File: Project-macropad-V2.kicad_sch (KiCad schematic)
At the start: 50 parts, among them J1 Conn_01x04_Male, SW1 RotaryEncoder_Switch, SW2 SW_Push, SW3 SW_SPDT

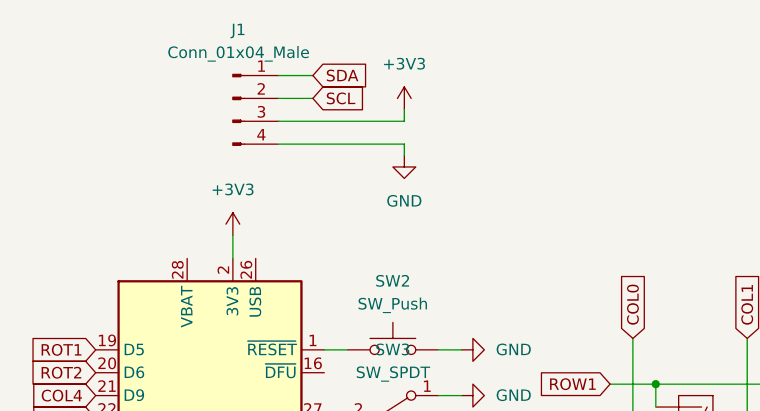
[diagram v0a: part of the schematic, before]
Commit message: Finished PCB
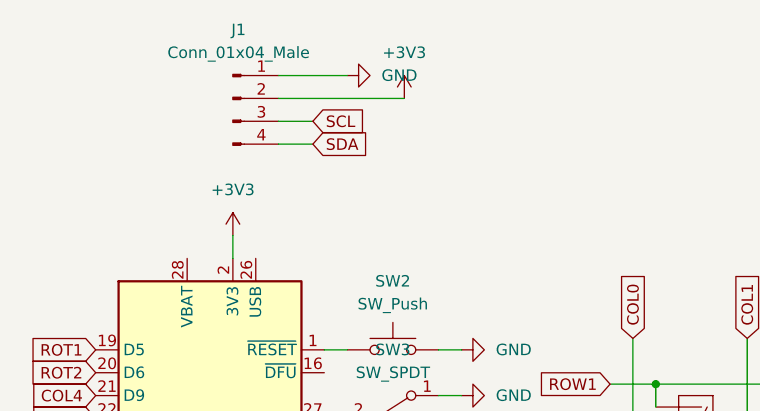
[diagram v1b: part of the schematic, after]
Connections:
- net +3V3: now also J1.2 (Pin_2); no longer J1.3 (Pin_3)
- net GND: now also J1.1 (Pin_1); no longer J1.4 (Pin_4)
- net SCL: now also J1.3 (Pin_3); no longer J1.2 (Pin_2)
- net SDA: now also J1.4 (Pin_4); no longer J1.1 (Pin_1)
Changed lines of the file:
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@@
-    (stroke (width 0) (type default) (color 0 0 0 0))
-  )
-  (wire (pts (xy 82.55 34.29) (xy 82.55 33.02))
     (stroke (width 0) (type default) (color 0 0 0 0))
   )
@@
     (stroke (width 0) (type default) (color 0 0 0 0))
   )
-  (wire (pts (xy 68.58 33.02) (xy 82.55 33.02))
-    (stroke (width 0) (type default) (color 0 0 0 0))
-  )
   (wire (pts (xy 135.89 125.73) (xy 135.89 128.27))
     (stroke (width 0) (type default) (color 0 0 0 0))
@@
     (stroke (width 0) (type default) (color 0 0 0 0))
   )
-  (wire (pts (xy 68.58 25.4) (xy 72.39 25.4))
-    (stroke (width 0) (type default) (color 0 0 0 0))
-  )
   (wire (pts (xy 110.49 78.74) (xy 110.49 76.2))
     (stroke (width 0) (type default) (color 0 0 0 0))
@@
     (stroke (width 0) (type default) (color 0 0 0 0))
   )
+  (wire (pts (xy 68.58 33.02) (xy 72.39 33.02))
+    (stroke (width 0) (type default) (color 0 0 0 0))
+  )
   (wire (pts (xy 115.57 67.31) (xy 109.22 67.31))
     (stroke (width 0) (type default) (color 0 0 0 0))
@@
     (stroke (width 0) (type default) (color 0 0 0 0))
   )
+  (wire (pts (xy 68.58 25.4) (xy 76.2 25.4))
+    (stroke (width 0) (type default) (color 0 0 0 0))
+  )
   (wire (pts (xy 123.19 92.71) (xy 135.89 92.71))
     (stroke (width 0) (type default) (color 0 0 0 0))
@@
     (stroke (width 0) (type default) (color 0 0 0 0))
   )
+  (wire (pts (xy 68.58 27.94) (xy 82.55 27.94))
+    (stroke (width 0) (type default) (color 0 0 0 0))
+  )
   (wire (pts (xy 115.57 128.27) (xy 115.57 125.73))
     (stroke (width 0) (type default) (color 0 0 0 0))
@@
     (stroke (width 0) (type default) (color 0 0 0 0))
   )
-  (wire (pts (xy 68.58 27.94) (xy 72.39 27.94))
-    (stroke (width 0) (type default) (color 0 0 0 0))
-  )
   (wire (pts (xy 128.27 83.82) (xy 121.92 83.82))
     (stroke (width 0) (type default) (color 0 0 0 0))
@@
     (stroke (width 0) (type default) (color 0 0 0 0))
   )
+  (wire (pts (xy 68.58 30.48) (xy 72.39 30.48))
+    (stroke (width 0) (type default) (color 0 0 0 0))
+  )
   (wire (pts (xy 135.89 59.69) (xy 148.59 59.69))
     (stroke (width 0) (type default) (color 0 0 0 0))
@@
     (stroke (width 0) (type default) (color 0 0 0 0))
   )
-  (wire (pts (xy 68.58 30.48) (xy 82.55 30.48))
-    (stroke (width 0) (type default) (color 0 0 0 0))
-  )
   (wire (pts (xy 158.75 88.9) (xy 160.02 88.9))
     (stroke (width 0) (type default) (color 0 0 0 0))
   )
-  (wire (pts (xy 82.55 30.48) (xy 82.55 29.21))
-    (stroke (width 0) (type default) (color 0 0 0 0))
-  )
   (wire (pts (xy 153.67 67.31) (xy 147.32 67.31))
     (stroke (width 0) (type default) (color 0 0 0 0))
@@
     )
   )
-  (global_label "SDA" (shape input) (at 72.39 25.4 0) (fields_autoplaced)
-    (effects (font (size 1.27 1.27)) (justify left))
-    (property "Intersheet References" "${INTERSHEET_REFS}" (id 0) (at 78.3712 25.3206 0)
+  (global_label "SDA" (shape input) (at 72.39 33.02 0) (fields_autoplaced)
+    (effects (font (size 1.27 1.27)) (justify left))
+    (property "Intersheet References" "${INTERSHEET_REFS}" (id 0) (at 78.3712 32.9406 0)
       (effects (font (size 1.27 1.27)) (justify left) hide)
     )
@@
     )
   )
-  (global_label "SCL" (shape input) (at 72.39 27.94 0) (fields_autoplaced)
-    (effects (font (size 1.27 1.27)) (justify left))
-    (property "Intersheet References" "${INTERSHEET_REFS}" (id 0) (at 78.3107 27.8606 0)
+  (global_label "SCL" (shape input) (at 72.39 30.48 0) (fields_autoplaced)
+    (effects (font (size 1.27 1.27)) (justify left))
+    (property "Intersheet References" "${INTERSHEET_REFS}" (id 0) (at 78.3107 30.4006 0)
       (effects (font (size 1.27 1.27)) (justify left) hide)
     )
@@
     (pin "1")
   )
-  (symbol (lib_id "power:+3V3") (at 82.55 29.21 0) (unit 1)
-    (in_bom yes) (on_board yes) (fields_autoplaced)
-    (property "Reference" "#PWR0106" (id 0) (at 82.55 33.02 0)
-      (effects (font (size 1.27 1.27)) hide)
-    )
-    (property "Value" "+3V3" (id 1) (at 82.55 24.13 0))
-    (property "Footprint" "" (id 2) (at 82.55 29.21 0)
-      (effects (font (size 1.27 1.27)) hide)
-    )
-    (property "Datasheet" "" (id 3) (at 82.55 29.21 0)
+  (symbol (lib_id "power:+3V3") (at 82.55 27.94 0) (unit 1)
+    (in_bom yes) (on_board yes) (fields_autoplaced)
+    (property "Reference" "#PWR0106" (id 0) (at 82.55 31.75 0)
+      (effects (font (size 1.27 1.27)) hide)
+    )
+    (property "Value" "+3V3" (id 1) (at 82.55 22.86 0))
+    (property "Footprint" "" (id 2) (at 82.55 27.94 0)
+      (effects (font (size 1.27 1.27)) hide)
+    )
+    (property "Datasheet" "" (id 3) (at 82.55 27.94 0)
       (effects (font (size 1.27 1.27)) hide)
     )
@@
     (pin "2")
   )
-  (symbol (lib_id "power:GND") (at 82.55 34.29 0) (unit 1)
-    (in_bom yes) (on_board yes) (fields_autoplaced)
-    (property "Reference" "#PWR0105" (id 0) (at 82.55 40.64 0)
-      (effects (font (size 1.27 1.27)) hide)
-    )
-    (property "Value" "GND" (id 1) (at 82.55 39.37 0))
-    (property "Footprint" "" (id 2) (at 82.55 34.29 0)
-      (effects (font (size 1.27 1.27)) hide)
-    )
-    (property "Datasheet" "" (id 3) (at 82.55 34.29 0)
-      (effects (font (size 1.27 1.27)) hide)
-    )
+  (symbol (lib_id "power:GND") (at 76.2 25.4 90) (unit 1)
+    (in_bom yes) (on_board yes) (fields_autoplaced)
+    (property "Reference" "#PWR0105" (id 0) (at 82.55 25.4 0)
+      (effects (font (size 1.27 1.27)) hide)
+    )
+    (property "Value" "GND" (id 1) (at 80.01 25.3999 90)
+      (effects (font (size 1.27 1.27)) (justify right))
+    )
+    (property "Footprint" "" (id 2) (at 76.2 25.4 0)
+      (effects (font (size 1.27 1.27)) hide)
+    )
+    (property "Datasheet" "" (id 3) (at 76.2 25.4 0)
+      (effects (font (size 1.27 1.27)) hide)
+    )
